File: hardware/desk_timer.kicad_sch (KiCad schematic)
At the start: 14 parts, among them SW1 SW_Push, U1 STM32G0B1CBT6, Y1 32.768 KHz, 10ppm, 12.5pf, Y2 8 MHz, 10ppm, 10pf

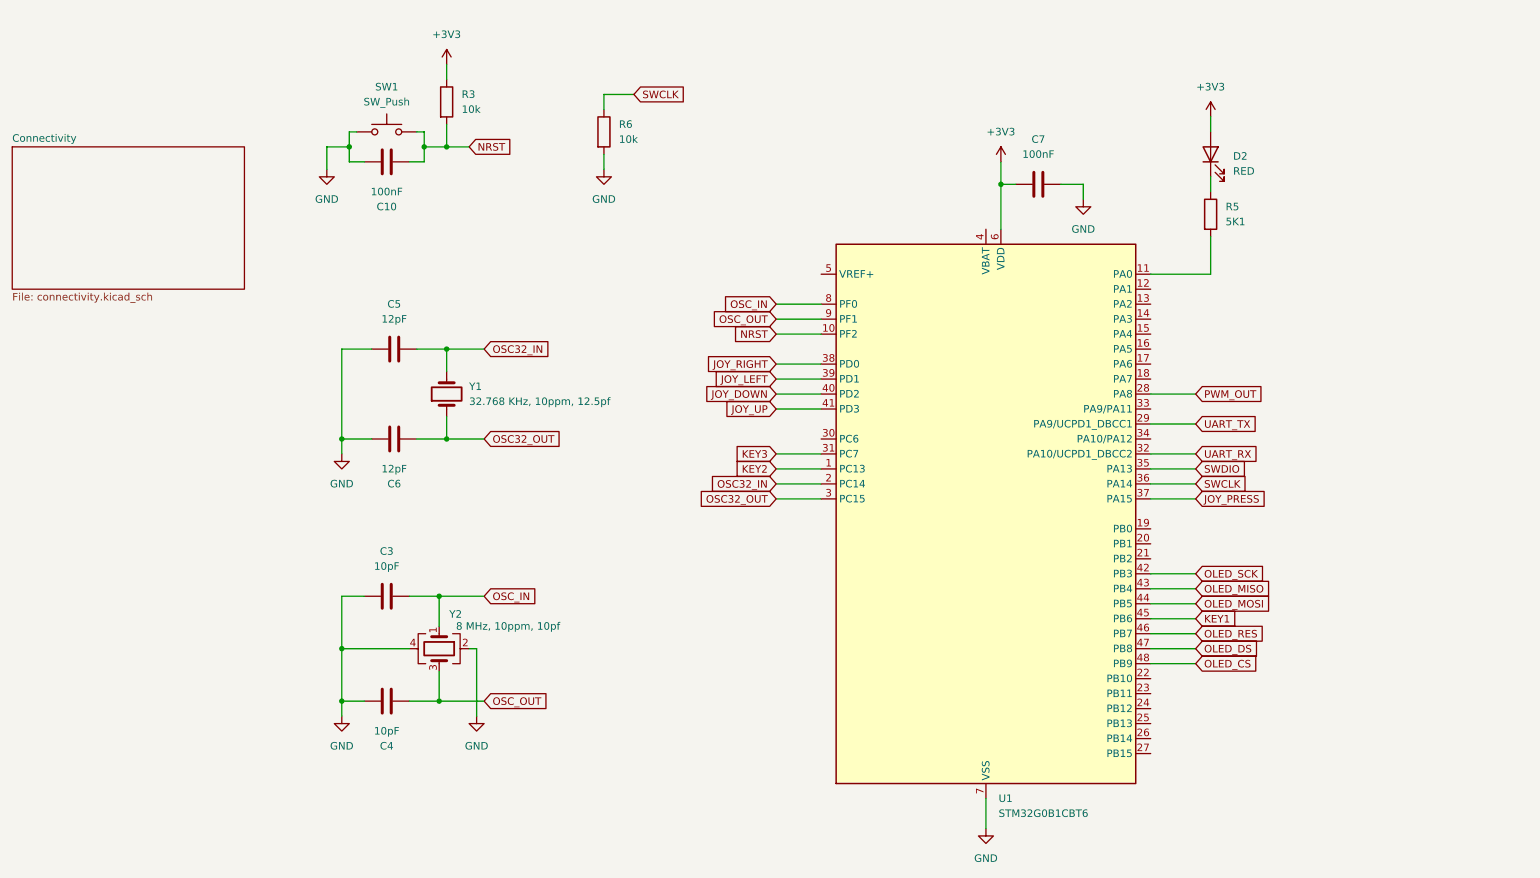
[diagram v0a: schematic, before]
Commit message: Finished board
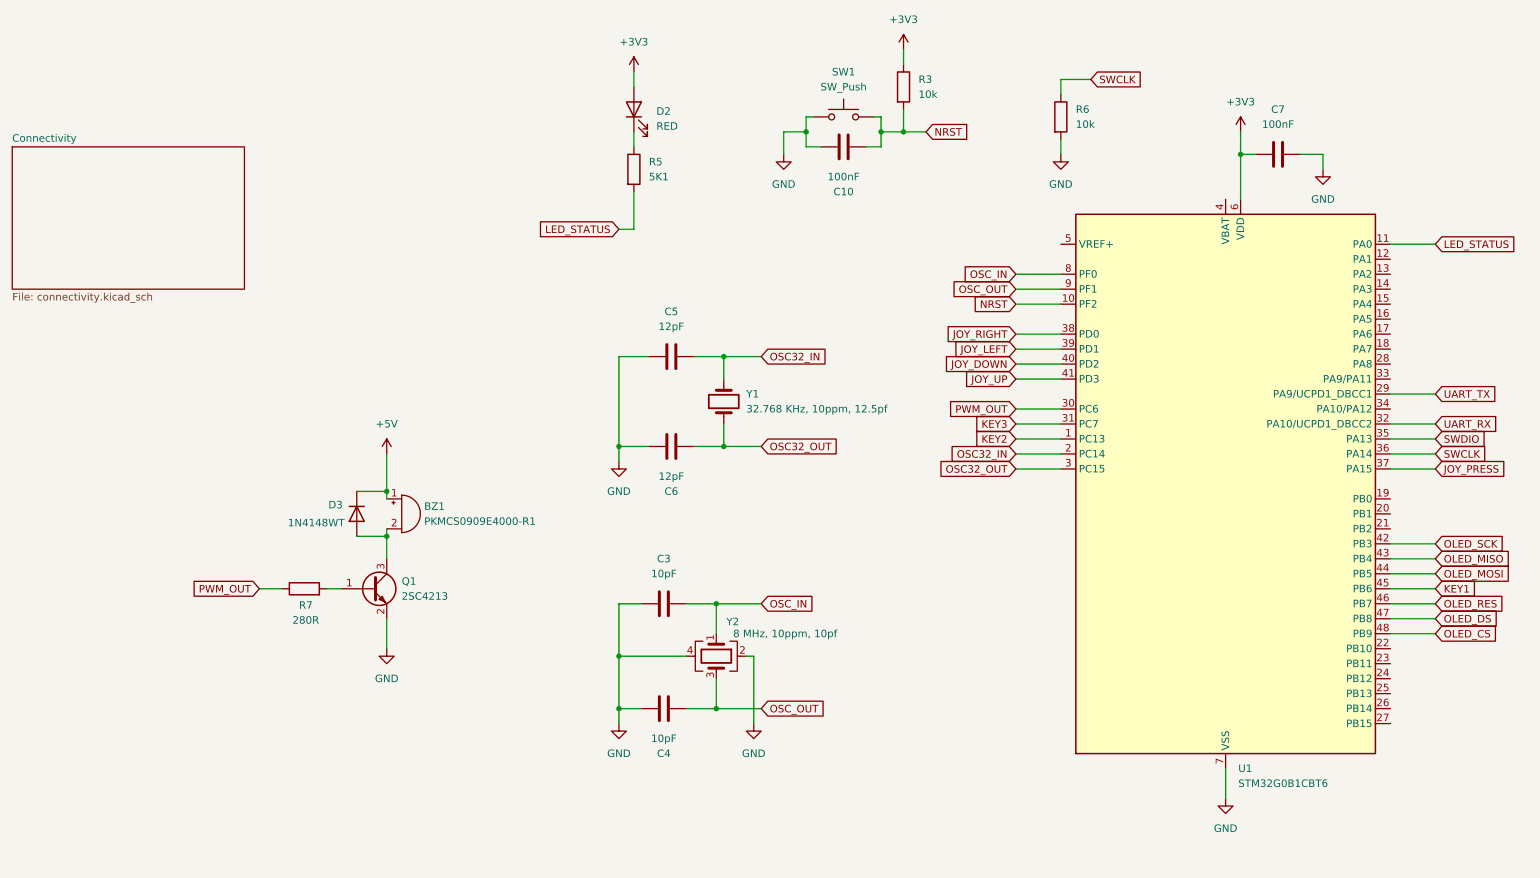
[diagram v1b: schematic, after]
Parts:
- added BZ1: PKMCS0909E4000-R1, Buzzer_Beeper:Buzzer_Murata_PKMCS0909E, symbol Device:Buzzer
- added D3: 1N4148WT, Diode_SMD:D_SOD-523, symbol Diode:1N4148WT
- added Q1: 2SC4213, Package_TO_SOT_SMD:SOT-323_SC-70, symbol Transistor_BJT:2SC4213
- added R7: 280R, Resistor_SMD:R_0402_1005Metric, symbol Device:R
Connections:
- net GND: now also Q1.2 (E)
- net PWM_OUT: now also U1.30 (PC6), R7.1; no longer U1.28 (PA8)
- net LED_STATUS: now reaches R5.2, U1.11 (PA0)
- new net: BZ1.2 (-), D3.2 (A), Q1.3 (C)
- new net: Q1.1 (B), R7.2
- new net +5V: BZ1.1 (+), D3.1 (K)
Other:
- moved on the sheet: C10, C3, C4, C5, C6, C7, D2, R3, R5, R6, SW1, U1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
